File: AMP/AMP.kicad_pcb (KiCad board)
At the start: 4 copper layers, 110 x 72 mm, 149 parts, among them J1 AudioJack4, J2 AudioJack4, J3 Screw_Terminal_01x02, J4 Barrel_Jack_MountingPin, U1 NE5532, U10 NE5532, U11 NE5532, U12 NE5532, U13 NE5532, U14 NE5532, U15 NE5532, U16 NE5532, U19 NE5532, U2 NE5532, U20 NE5532, U21 NE5532, U22 NE5532, U23 NE5532, U24 NE5532, U25 NE5532, U3 NE5532, U4 NE5532, U5 NE5532, U6 NE5532, U7 NE5532, U8 NE5532

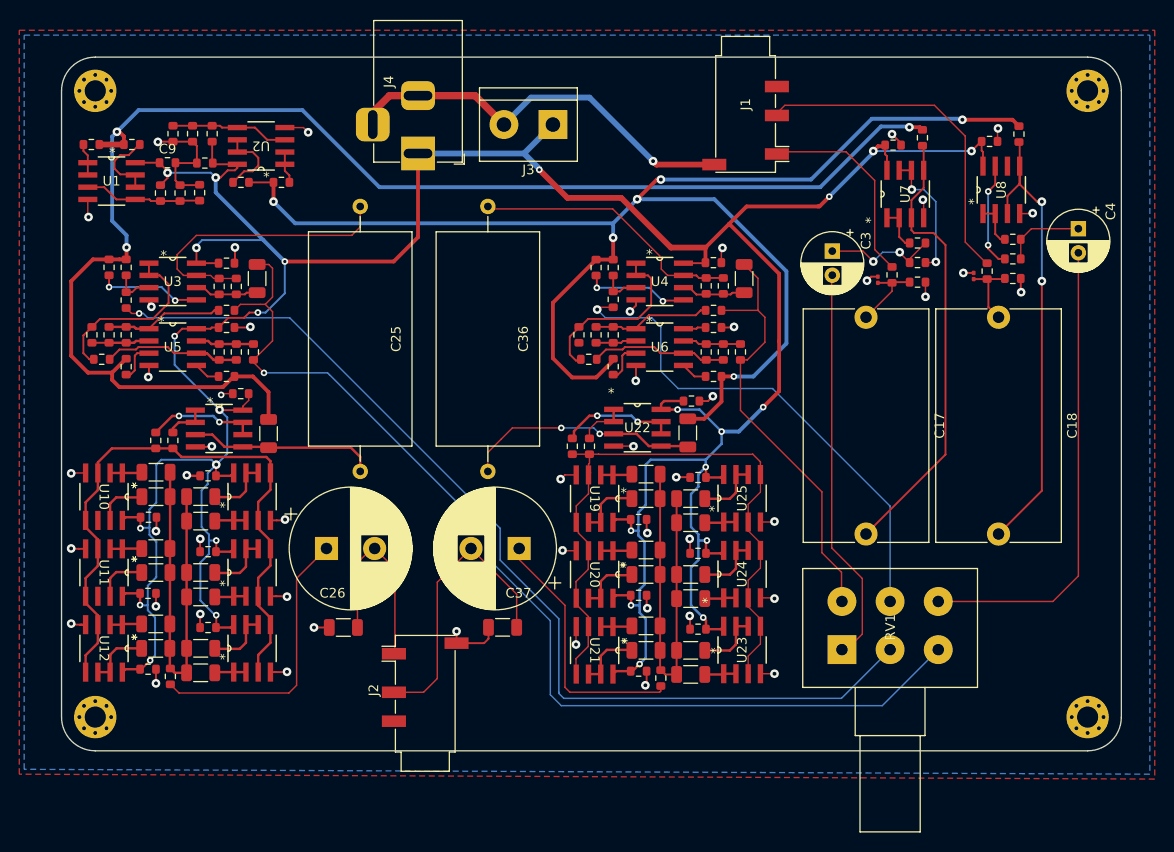
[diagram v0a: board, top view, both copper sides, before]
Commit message: updated files
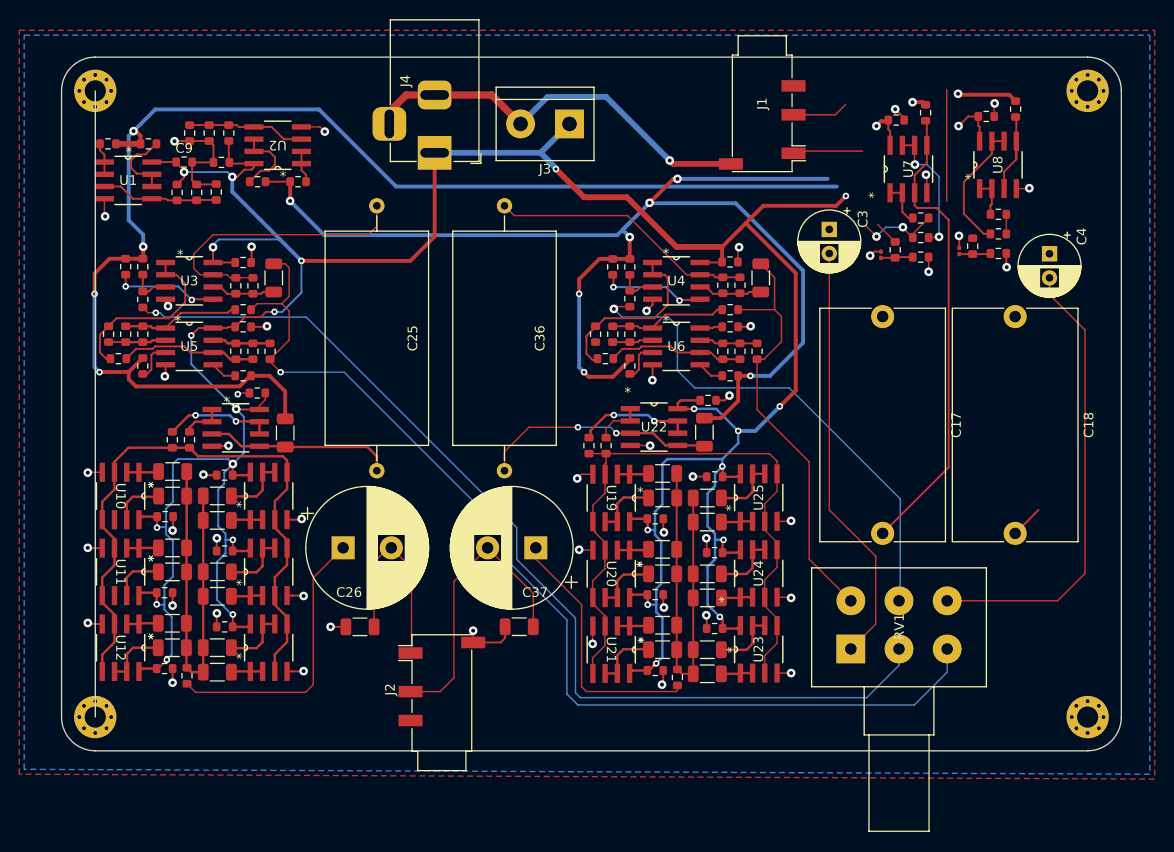
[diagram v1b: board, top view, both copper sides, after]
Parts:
- moved C4 3.97 mm to (177.5, 68.4)
- moved C20 3.00 mm to (168.2, 68.1)
- moved R34 3.00 mm to (169.6, 67.6)
- moved R38 3.00 mm to (172.2, 64.3)
- moved R40 3.00 mm to (172.2, 68.4)
- moved R42 3.00 mm to (172.2, 66.3)
- moved C24 2.62 mm to (171.0, 54.2)
- moved R32 2.62 mm to (174.0, 53.4)
- moved U8 2.62 mm to (172.2, 59.2)
- moved C19 2.62 mm to (160.1, 68.5)
- moved C23 2.62 mm to (161.6, 54.5)
- moved R33 2.62 mm to (161.5, 68.0)
- moved R37 2.62 mm to (164.2, 64.7)
- moved R39 2.62 mm to (164.2, 68.8)
- moved R41 2.62 mm to (164.2, 66.7)
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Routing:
- net Net-(C18-Pad2): track 49.3 -> 13.3 mm, vias 2 -> 0
- net RIGHT_AUDIO_IN: track 35.4 -> 17.5 mm
- net VBIAS_R: track 154.4 -> 138.1 mm, vias 6 -> 8
- net +15V: track 365.4 -> 349.7 mm
- net VBIAS_L: track 151.8 -> 139.8 mm, vias 3 -> 5
- net LEFT_AUDIO_IN: track 21.1 -> 9.72 mm
- net RIGHT_BUF_AUDIO: track 8.47 -> 2.03 mm
- net Net-(C17-Pad1): track 8.02 -> 3.33 mm
- net Net-(C18-Pad1): track 7.72 -> 3.45 mm
- net L_Pot1: track 41.4 -> 44.6 mm
- net LEFT_BUF_AUDIO: track 12.1 -> 8.88 mm
- net Net-(R42-Pad1): track 11.1 -> 13.7 mm, vias 2 -> 0
- net Net-(C17-Pad2): track 46.9 -> 48.9 mm
- net R_Pot1: track 49.2 -> 47.7 mm
- net VOL_OUT_R: track 28.2 -> 27.5 mm
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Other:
- outline, holes or cut-outs redrawn
